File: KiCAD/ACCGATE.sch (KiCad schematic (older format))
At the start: 58 parts

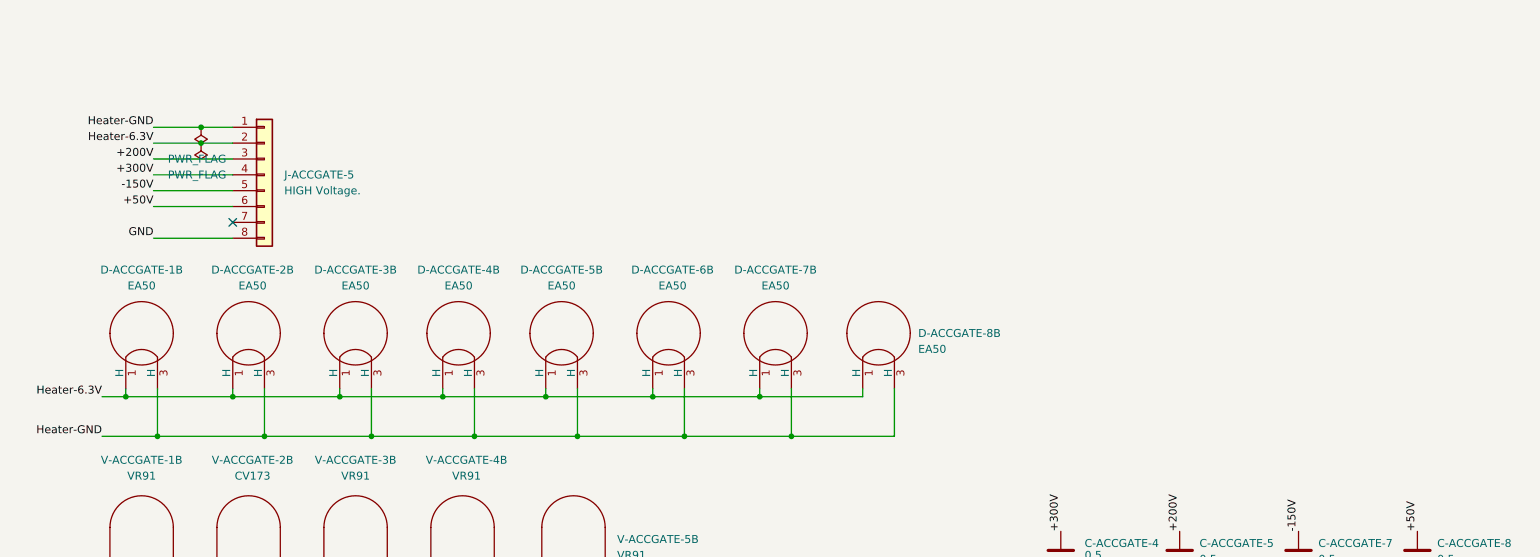
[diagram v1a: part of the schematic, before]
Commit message: Add scfollws.sch
Signed-off-by: John Bradley <flypie@rocketmail.com>
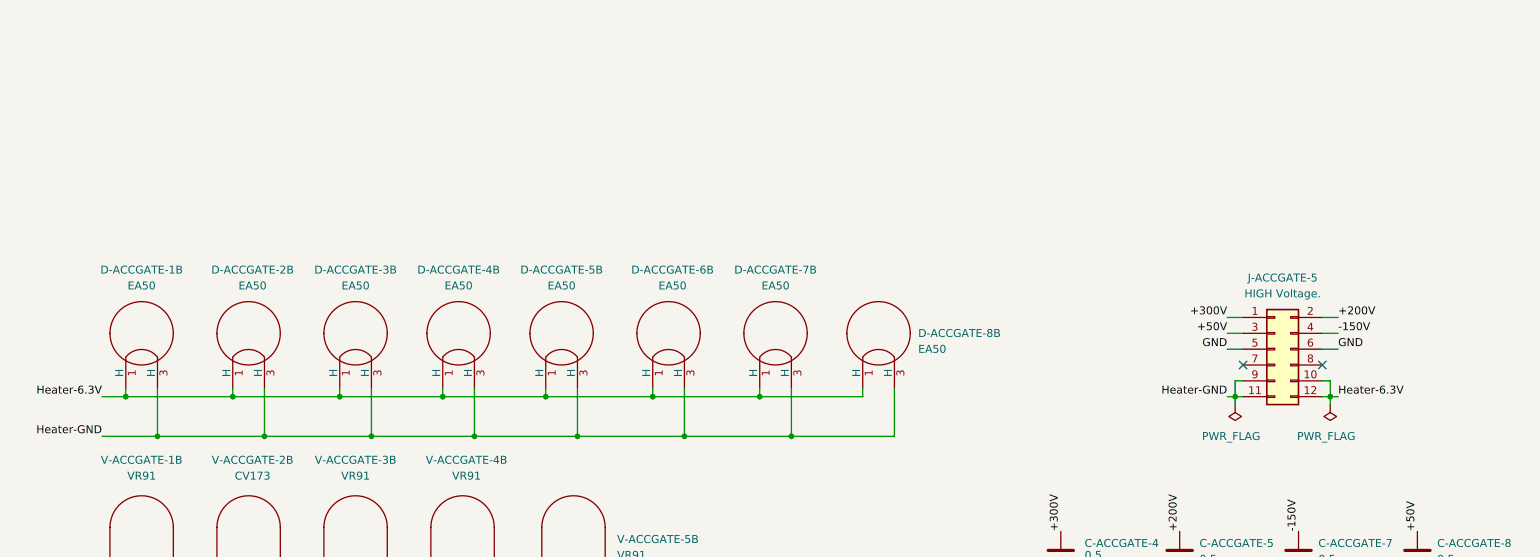
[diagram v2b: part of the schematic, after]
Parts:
- removed J-ACCGATE-5: HIGH Voltage., Connector_TE-Connectivity:TE_MATE-N-LOK_1-770970-x_2x04_P4.14mm_Horizontal, symbol Connector_Generic:Conn_01x08
- added J-ACCGATE-5: HIGH Voltage., Connector_TE-Connectivity:TE_MATE-N-LOK_1-770972-x_2x06_P4.14mm_Horizontal, symbol Connector_Generic:Conn_02x06_Odd_Even
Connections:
- net +200V: now also J-ACCGATE-5.2 (Pin_2)
- net +300V: now also J-ACCGATE-5.1 (Pin_1)
- net +50V: now also J-ACCGATE-5.3 (Pin_3)
- net -150V: now also J-ACCGATE-5.4 (Pin_4)
- net GND: now also J-ACCGATE-5.5 (Pin_5), J-ACCGATE-5.6 (Pin_6)
- net Heater-6.3V: now also J-ACCGATE-5.10 (Pin_10), J-ACCGATE-5.12 (Pin_12)
- net Heater-GND: now also J-ACCGATE-5.11 (Pin_11), J-ACCGATE-5.9 (Pin_9)
- no-connect marks 11 -> 12
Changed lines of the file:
@@
 $Descr A3 16535 11693
 encoding utf-8
-Sheet 8 32
+Sheet 8 33
 Title "Control Gate Posn 6.3"
 Date "2020-10-08"
@@
 Text Label 4325 2625 1    50   ~ 0
 +300V
-Wire Wire Line
-	2125 7950 1925 7950
-Wire Wire Line
-	2125 7850 1925 7850
-$Comp
-L power:PWR_FLAG #FLG0115
-U 1 1 6064965D
-P 1925 7950
-F 0 "#FLG0115" H 1925 8025 50  0001 C CNN
-F 1 "PWR_FLAG" H 1950 8150 50  0000 C CNN
-F 2 "" H 1925 7950 50  0001 C CNN
-F 3 "~" H 1925 7950 50  0001 C CNN
-	1    1925 7950
-	-1   0    0    1
-$EndComp
-$Comp
-L power:PWR_FLAG #FLG0116
-U 1 1 5FE97B82
-P 1925 7850
-F 0 "#FLG0116" H 1925 7925 50  0001 C CNN
-F 1 "PWR_FLAG" H 1950 8050 50  0000 C CNN
-F 2 "" H 1925 7850 50  0001 C CNN
-F 3 "~" H 1925 7850 50  0001 C CNN
-	1    1925 7850
-	-1   0    0    1
-$EndComp
-Connection ~ 1925 7850
-Wire Wire Line
-	1925 7850 1625 7850
-Wire Wire Line
-	2125 8050 1625 8050
-Wire Wire Line
-	2125 8150 1625 8150
-Wire Wire Line
-	2125 8350 1625 8350
-$Comp
-L Connector_Generic:Conn_01x08 J-ACCGATE-5
-U 1 1 6064965F
-P 2325 8150
-F 0 "J-ACCGATE-5" H 2450 8150 50  0000 L CNN
-F 1 "HIGH Voltage." H 2450 8050 50  0000 L CNN
-F 2 "Connector_TE-Connectivity:TE_MATE-N-LOK_1-770970-x_2x04_P4.14mm_Horizontal" H 2325 8150 50  0001 C CNN
-F 3 "~" H 2325 8150 50  0001 C CNN
-	1    2325 8150
-	1    0    0    -1
-$EndComp
-Connection ~ 1925 7950
-Wire Wire Line
-	1925 7950 1625 7950
-NoConn ~ 2125 8450
-Text Label 1625 7850 2    50   ~ 0
-Heater-GND
-Text Label 1625 7950 2    50   ~ 0
-Heater-6.3V
-Text Label 1625 8050 2    50   ~ 0
-+200V
-Text Label 1625 8150 2    50   ~ 0
-+300V
-Text Label 1625 8250 2    50   ~ 0
--150V
-Text Label 1625 8350 2    50   ~ 0
-+50V
 Text Label 1300 9550 2    50   ~ 0
 Heater-6.3V
@@
 Text Label 1300 11175 2    50   ~ 0
 Heater-GND
-Text Label 1625 8550 2    50   ~ 0
-GND
 Text Label 4325 4225 3    50   ~ 0
 GND
@@
 Text Label 6950 4225 2    50   ~ 0
 GND
-Wire Wire Line
-	1625 8550 2125 8550
 $Comp
 L Connector:Conn_01x01_Female J-ACCGATE-6
@@
 Text Label 8850 10800 3    50   ~ 0
 GND
-Wire Wire Line
-	1625 8250 2125 8250
 Text Label 7350 10400 1    50   ~ 0
 +300V
@@
 	1    0    0    -1
 $EndComp
+$Comp
+L power:PWR_FLAG #FLG?
+U 1 1 60B39D71
+P 9050 9600
+AR Path="/5F868E46/60B39D71" Ref="#FLG?"  Part="1"
+AR Path="/5F2DDAEA/60B39D71" Ref="#FLG0115"  Part="1"
+F 0 "#FLG0115" H 9050 9675 50  0001 C CNN
+F 1 "PWR_FLAG" H 9075 9800 50  0000 C CNN
+F 2 "" H 9050 9600 50  0001 C CNN
+F 3 "~" H 9050 9600 50  0001 C CNN
+	1    9050 9600
+	-1   0    0    1
+$EndComp
+$Comp
+L Connector_Generic:Conn_02x06_Odd_Even J-SCFOLLWS-?
+U 1 1 60B39D77
+P 8700 9250
+AR Path="/5F868E46/60B39D77" Ref="J-SCFOLLWS-?"  Part="1"
+AR Path="/5F2DDAEA/60B39D77" Ref="J-ACCGATE-5"  Part="1"
+F 0 "J-ACCGATE-5" H 8750 9700 50  0000 C CNN
+F 1 "HIGH Voltage." H 8750 9600 50  0000 C CNN
+F 2 "Connector_TE-Connectivity:TE_MATE-N-LOK_1-770972-x_2x06_P4.14mm_Horizontal" H 8700 9250 50  0001 C CNN
+F 3 "~" H 8700 9250 50  0001 C CNN
+	1    8700 9250
+	1    0    0    -1
+$EndComp
+Text Label 8400 9050 2    50   ~ 0
++300V
+Text Label 9100 9150 0    50   ~ 0
+-150V
+Text Label 8400 9150 2    50   ~ 0
++50V
+Text Label 8400 9250 2    50   ~ 0
+GND
+NoConn ~ 8500 9350
+$Comp
+L power:PWR_FLAG #FLG?
+U 1 1 60B39D82
+P 8450 9600
+AR Path="/5F868E46/60B39D82" Ref="#FLG?"  Part="1"
+AR Path="/5F2DDAEA/60B39D82" Ref="#FLG0116"  Part="1"
+F 0 "#FLG0116" H 8450 9675 50  0001 C CNN
+F 1 "PWR_FLAG" H 8475 9800 50  0000 C CNN
+F 2 "" H 8450 9600 50  0001 C CNN
+F 3 "~" H 8450 9600 50  0001 C CNN
+	1    8450 9600
+	-1   0    0    1
+$EndComp
+Wire Wire Line
+	8500 9550 8450 9550
+Wire Wire Line
+	8450 9600 8450 9550
+Connection ~ 8450 9550
+Wire Wire Line
+	8450 9550 8400 9550
+Wire Wire Line
+	9000 9550 9050 9550
+Text Label 9100 9550 0    50   ~ 0
+Heater-6.3V
+Connection ~ 9050 9550
+Wire Wire Line
+	9050 9550 9100 9550
+Wire Wire Line
+	9100 9050 9000 9050
+Wire Wire Line
+	9100 9150 9000 9150
+Wire Wire Line
+	9100 9250 9000 9250
+Wire Wire Line
+	8500 9050 8400 9050
+Wire Wire Line
+	8500 9150 8400 9150
+Wire Wire Line
+	8500 9250 8400 9250
+Wire Wire Line
+	8450 9550 8450 9450
+Wire Wire Line
+	8450 9450 8500 9450
+Wire Wire Line
+	9050 9550 9050 9450
+Wire Wire Line
+	9050 9450 9000 9450
+Wire Wire Line
+	9050 9600 9050 9550
+Text Label 9100 9050 0    50   ~ 0
++200V
+Text Label 9100 9250 0    50   ~ 0
+GND
+NoConn ~ 9000 9350
+Text Label 8400 9550 2    50   ~ 0
+Heater-GND
 $EndSCHEMATC

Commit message: Add sclock correct fault in ACGATE.
Signed-off-by: John Bradley <flypie@rocketmail.com>
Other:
- moved on the sheet: C-ACCGATE-2, C-ACCGATE-3, C-ACCGATE-6, D-ACCGATE-1A, D-ACCGATE-2A, D-ACCGATE-3A, D-ACCGATE-4A, D-ACCGATE-7A, J-ACCGATE-10, J-ACCGATE-11, J-ACCGATE-12, J-ACCGATE-13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
